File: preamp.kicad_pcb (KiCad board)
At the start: 2 copper layers, 39 parts, among them J1 JACK_TRS_6PINS, J2 JACK_TRS_6PINS, P1 CONN_01X02, P2 RCA_L, P3 RCA_R, U1 NE5532

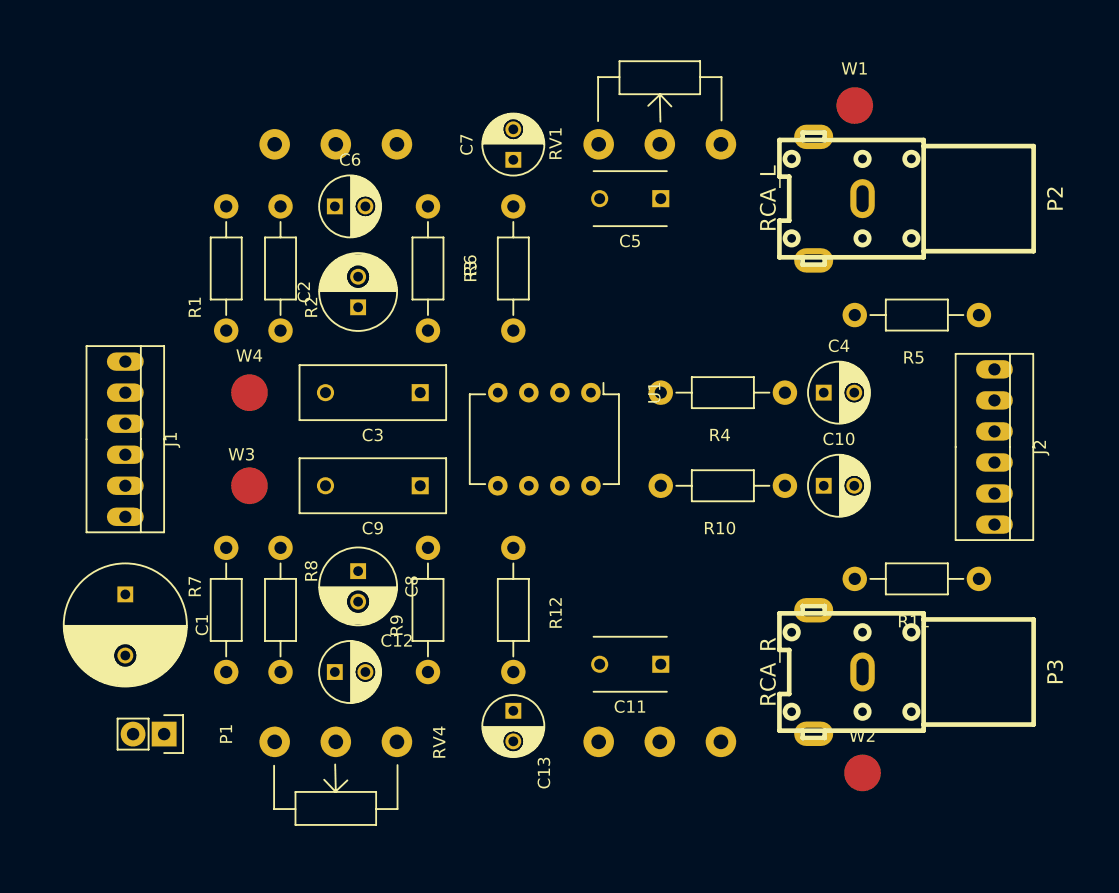
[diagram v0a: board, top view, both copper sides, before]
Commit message: pcb roteada
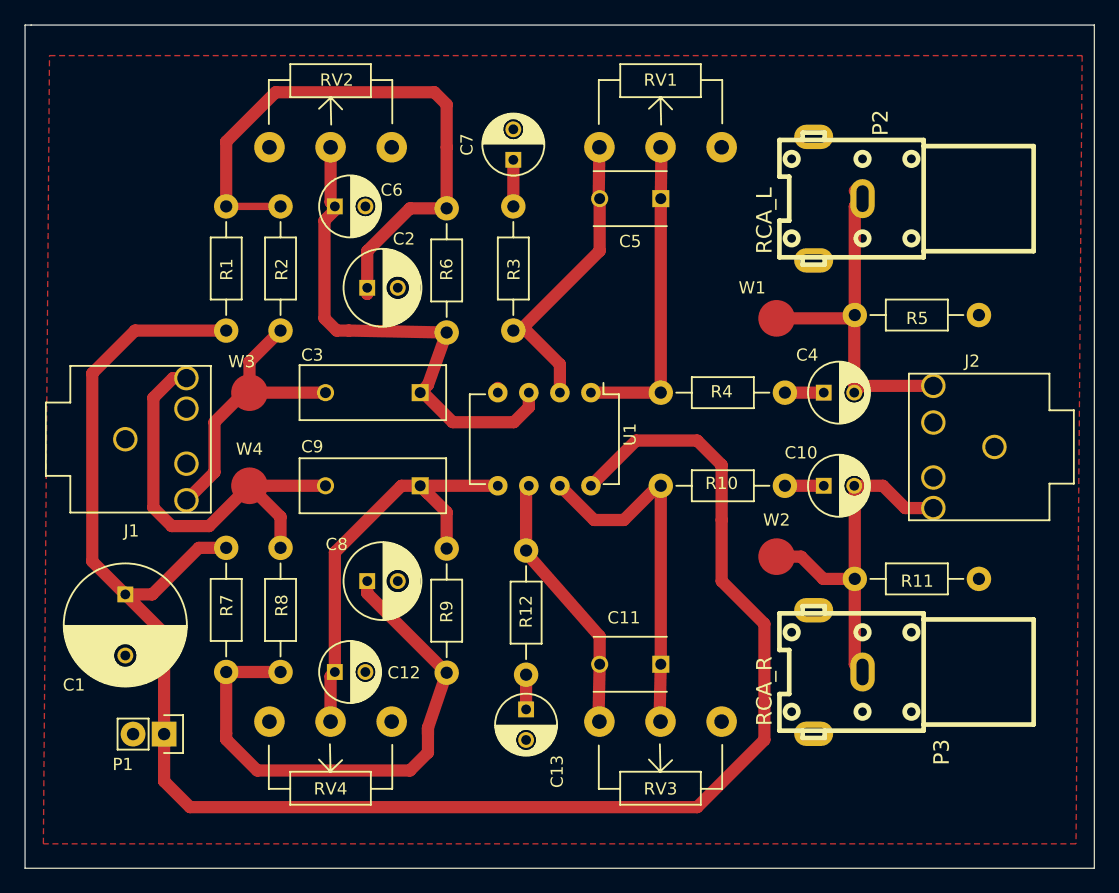
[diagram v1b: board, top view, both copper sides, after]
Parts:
- J1, J2: value JACK_TRS_6PINS -> JACK_STEREO; footprint Connect:PINHEAD1-6 -> audio_conn:audio_jack
- RV2, RV3: moved to F.Cu
- moved W2 19.0 mm to (169.5, 82.0)
- moved W1 18.6 mm to (169.5, 62.5)
- moved RV2 10.4 mm to (128.0, 48.5)
- moved RV3 10.2 mm to (165.0, 95.5)
- moved W3 7.62 mm to (126.4, 68.6)
- moved W4 7.62 mm to (126.4, 76.2)
- moved C2 1.76 mm to (136.0, 60.0), turned to 0 degrees
- moved RV4 1.71 mm to (138.0, 95.5)
- moved R3 1.54 mm to (142.5, 53.5)
- moved R9 1.53 mm to (142.5, 91.5)
- moved C8 1.10 mm to (136.0, 84.0), turned to 0 degrees
- moved R12 1.07 mm to (149.0, 81.5)
- moved C13 1.05 mm to (149.0, 94.5)
- moved RV1 0.25 mm to (155.0, 48.5)
- turned J1 to 0 degrees
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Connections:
- RV1 pad 3: Net-(RV1-Pad3) -> (no net)
- RV2 pad 1: GND -> (no net)
- RV2 pad 3: Net-(RV2-Pad3) -> GND
- RV3 pad 1: Net-(C11-Pad2) -> (no net)
- RV3 pad 3: Net-(RV3-Pad3) -> Net-(C11-Pad2)
- RV4 pad 3: Net-(RV4-Pad3) -> (no net)
- W3 pad 1: /R_IN -> /L_IN
- W4 pad 1: /L_IN -> /R_IN
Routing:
- net +9V: track 0.00 -> 147.3 mm
- net Net-(C2-Pad1): track 0.00 -> 50.3 mm
- net Net-(C8-Pad1): track 0.00 -> 45.6 mm
- net Net-(C3-Pad1): track 0.00 -> 42.0 mm
- net Net-(C12-Pad1): track 0.00 -> 36.5 mm
- net /R_IN: track 0.00 -> 34.9 mm
- net /L_OUT: track 0.00 -> 30.3 mm
- net Net-(C11-Pad1): track 0.00 -> 29.9 mm
- net /R_OUT: track 0.00 -> 29.9 mm
- net Net-(C5-Pad1): track 0.00 -> 25.8 mm
- net Net-(C5-Pad2): track 0.00 -> 25.5 mm
- net /L_IN: track 0.00 -> 25.0 mm
- net Net-(C11-Pad2): track 0.00 -> 21.7 mm
- net Net-(C7-Pad1): track 0.00 -> 3.81 mm
- net Net-(C4-Pad1): track 0.00 -> 3.17 mm
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- added copper zone on F.Cu, net GND
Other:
- board outline added: 87.5 x 69 mm
- net class Default: clearance 0.2 -> 0.254; trace_width 0.25 -> 0.3; via_dia 0.6 -> 2; via_drill 0.4 -> 1.5
- rule trace_clearance: 0.2 -> 0.254
- rule trace_min: 0.2 -> 0.3
- rule via_min_drill: 0.3 -> 1.5
- rule via_min_size: 0.4 -> 1.5
